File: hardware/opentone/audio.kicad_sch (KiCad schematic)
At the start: 36 parts

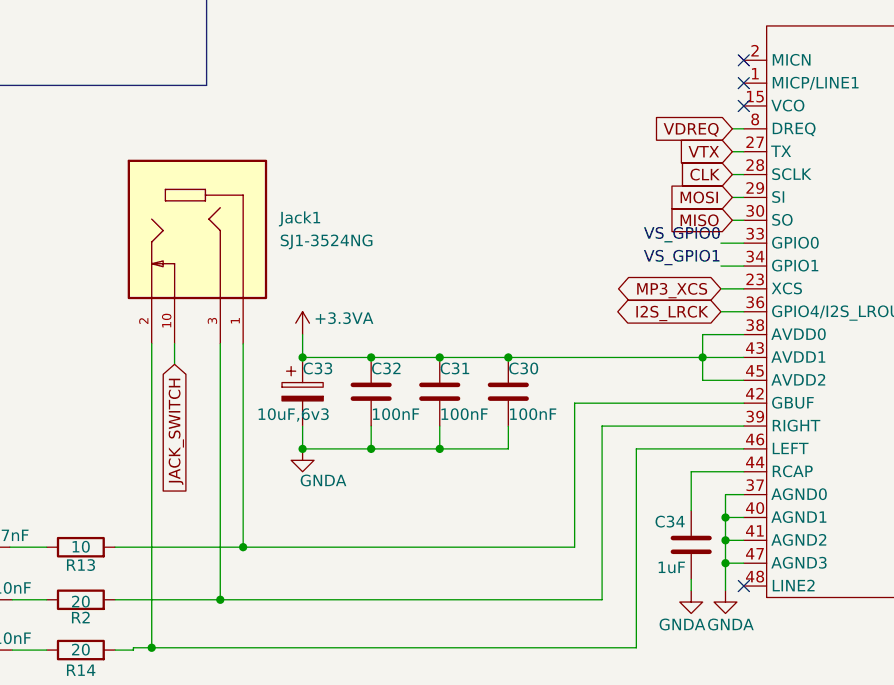
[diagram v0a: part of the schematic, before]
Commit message: wiring main MCU
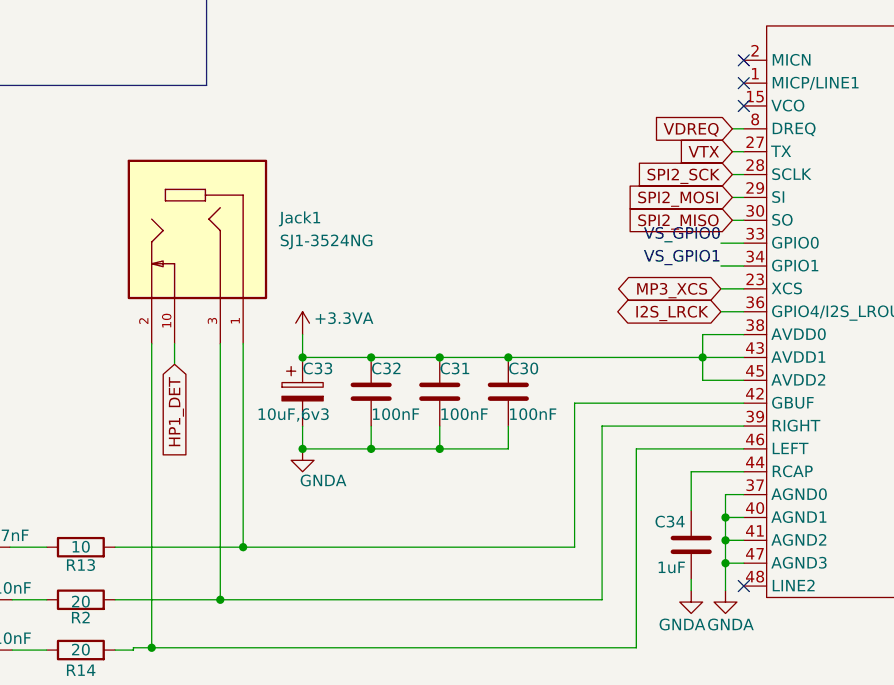
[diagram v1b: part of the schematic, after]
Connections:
- net CLK renamed SPI2_SCK
- net JACK_SWITCH renamed HP1_DET
- net MISO renamed SPI2_MISO
- net MOSI renamed SPI2_MOSI
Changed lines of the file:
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@@
 		)
 	)
-	(global_label "CLK"
+	(global_label "SPI2_SCK"
 		(shape input)
 		(at 134.112 63.5 180)
@@
 		)
 	)
-	(global_label "MOSI"
+	(global_label "SPI2_MOSI"
 		(shape input)
 		(at 134.112 66.04 180)
@@
 		)
 	)
-	(global_label "JACK_SWITCH"
+	(global_label "HP1_DET"
 		(shape input)
 		(at 72.136 84.582 270)
@@
 		)
 	)
-	(global_label "MISO"
+	(global_label "SPI2_MISO"
 		(shape input)
 		(at 134.112 68.58 180)
